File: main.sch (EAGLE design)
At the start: 4 parts, among them X1 1751248, X2 1751251

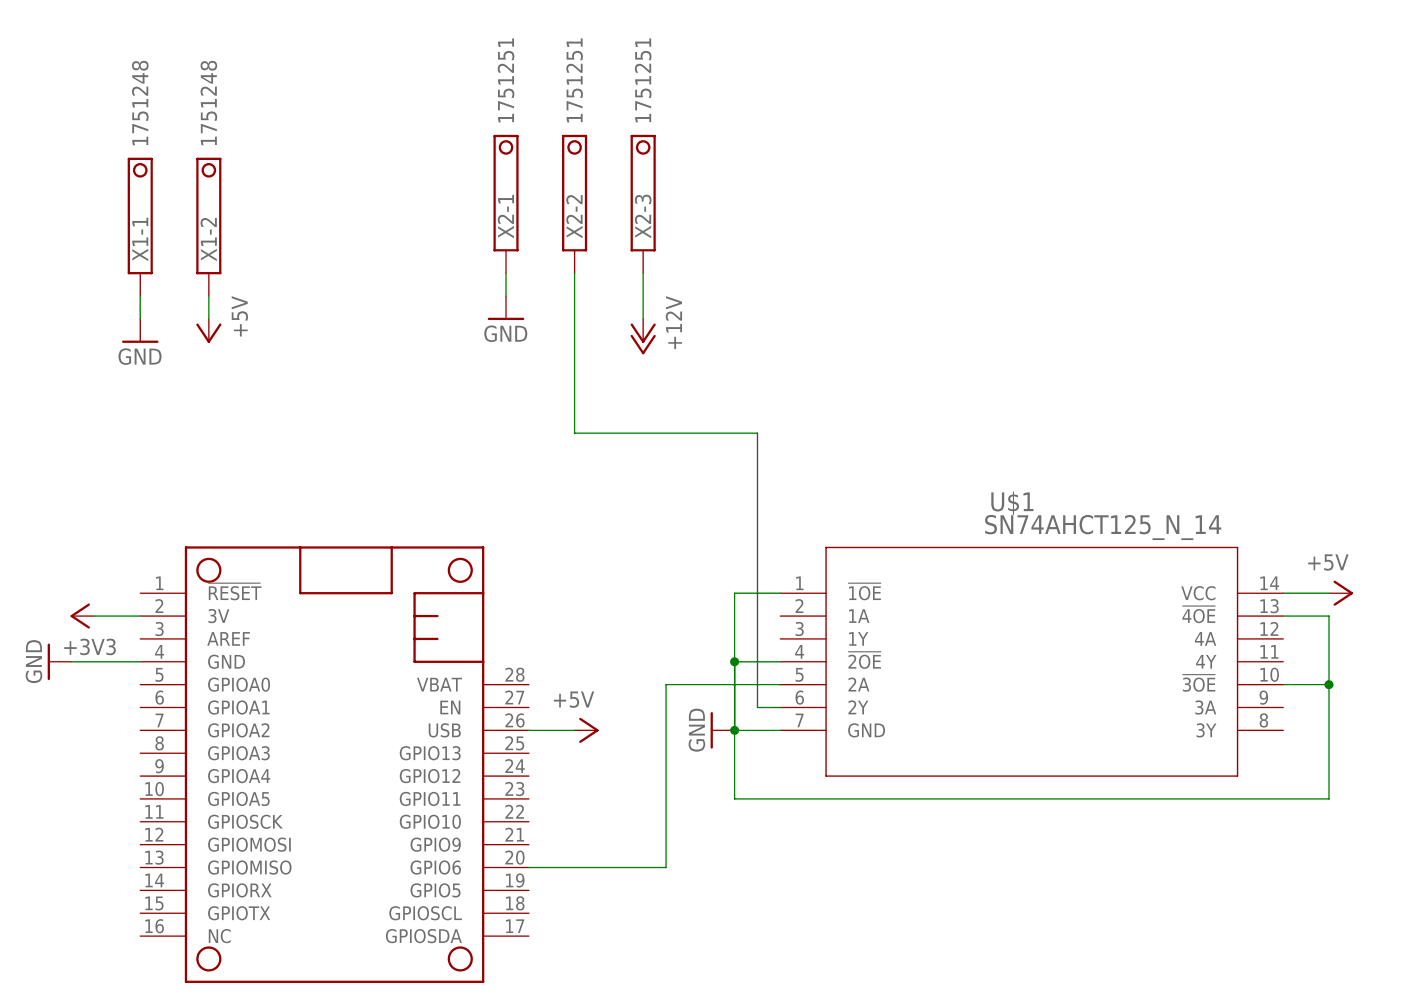
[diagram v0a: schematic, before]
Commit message: v2
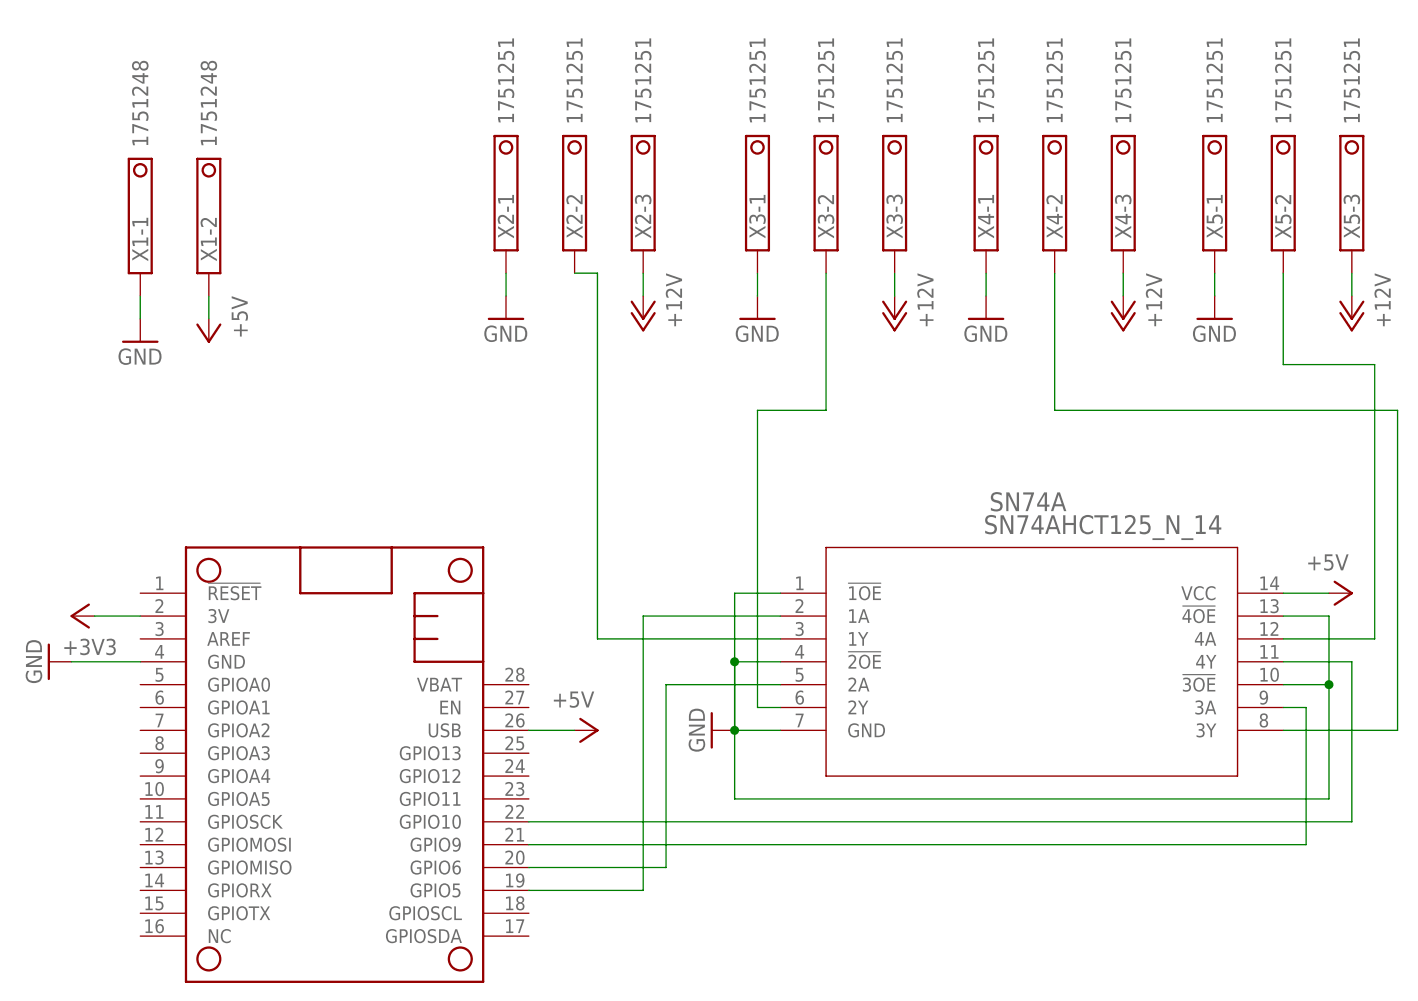
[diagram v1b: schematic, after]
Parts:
- added X3, X4, X5: 1751251, con-phoenix-350:1751251
- renumbered U$1 to SN74A
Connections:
- net LDATA renamed LDATA2
- removed net HDATA: SN74A.2Y, X2-2.K
- new net HDATA1: SN74A.1Y, X2-2.K
- new net HDATA2: SN74A.2Y, X3-2.K
- new net HDATA3: SN74A.3Y, X4-2.K
- new net HDATA4: SN74A.4A, X5-2.K
- new net LDATA1: MS1.GPIO5, SN74A.1A
- new net LDATA3: MS1.GPIO9, SN74A.3A
- new net LDATA4: MS1.GPIO10, SN74A.4Y
- net +12V: now also X3-3.K, X4-3.K, X5-3.K
- net GND: now also X3-1.K, X4-1.K, X5-1.K
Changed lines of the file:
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@@
 </variantdefs>
 <classes>
-<class number="0" name="default" width="0.381" drill="0">
+<class number="0" name="default" width="0.762" drill="0">
 <clearance class="0" value="0.3048"/>
 </class>
@@
 <parts>
 <part name="MS1" library="adafruit" deviceset="FEATHERWING" device="_NODIM"/>
-<part name="U$1" library="SN74AHCT125N" deviceset="SN74AHCT125_N_14" device=""/>
+<part name="SN74A" library="SN74AHCT125N" deviceset="SN74AHCT125_N_14" device=""/>
 <part name="GND2" library="supply1" deviceset="GND" device=""/>
 <part name="GND3" library="supply1" deviceset="GND" device=""/>
@@
 <part name="P+3" library="supply1" deviceset="+5V" device=""/>
 <part name="P+4" library="supply1" deviceset="+12V" device=""/>
+<part name="X3" library="con-phoenix-350" deviceset="1751251" device=""/>
+<part name="X4" library="con-phoenix-350" deviceset="1751251" device=""/>
+<part name="X5" library="con-phoenix-350" deviceset="1751251" device=""/>
+<part name="GND5" library="supply1" deviceset="GND" device=""/>
+<part name="GND6" library="supply1" deviceset="GND" device=""/>
+<part name="GND7" library="supply1" deviceset="GND" device=""/>
+<part name="P+5" library="supply1" deviceset="+12V" device=""/>
+<part name="P+6" library="supply1" deviceset="+12V" device=""/>
+<part name="P+7" library="supply1" deviceset="+12V" device=""/>
 </parts>
 <sheets>
@@
 <instances>
 <instance part="MS1" gate="G$1" x="-27.94" y="81.28" rot="R270"/>
-<instance part="U$1" gate="A" x="35.56" y="76.2"/>
+<instance part="SN74A" gate="A" x="35.56" y="76.2"/>
 <instance part="GND2" gate="1" x="-43.18" y="68.58" rot="R270"/>
 <instance part="GND3" gate="1" x="30.48" y="60.96" rot="R270"/>
@@
 <instance part="GND4" gate="1" x="7.62" y="106.68"/>
 <instance part="P+3" gate="1" x="101.6" y="76.2" rot="R270"/>
-<instance part="P+4" gate="1" x="22.86" y="104.14" rot="R180"/>
+<instance part="P+4" gate="1" x="22.86" y="106.68" rot="R180"/>
+<instance part="X3" gate="-1" x="35.56" y="114.3" rot="R90"/>
+<instance part="X3" gate="-2" x="43.18" y="114.3" rot="R90"/>
+<instance part="X3" gate="-3" x="50.8" y="114.3" rot="R90"/>
+<instance part="X4" gate="-1" x="60.96" y="114.3" rot="R90"/>
+<instance part="X4" gate="-2" x="68.58" y="114.3" rot="R90"/>
+<instance part="X4" gate="-3" x="76.2" y="114.3" rot="R90"/>
+<instance part="X5" gate="-1" x="86.36" y="114.3" rot="R90"/>
+<instance part="X5" gate="-2" x="93.98" y="114.3" rot="R90"/>
+<instance part="X5" gate="-3" x="101.6" y="114.3" rot="R90"/>
+<instance part="GND5" gate="1" x="35.56" y="106.68"/>
+<instance part="GND6" gate="1" x="60.96" y="106.68"/>
+<instance part="GND7" gate="1" x="86.36" y="106.68"/>
+<instance part="P+5" gate="1" x="50.8" y="106.68" rot="R180"/>
+<instance part="P+6" gate="1" x="76.2" y="106.68" rot="R180"/>
+<instance part="P+7" gate="1" x="101.6" y="106.68" rot="R180"/>
 </instances>
 <busses>
@@
 <segment>
 <pinref part="GND3" gate="1" pin="GND"/>
-<pinref part="U$1" gate="A" pin="GND"/>
+<pinref part="SN74A" gate="A" pin="GND"/>
 <wire x1="33.02" y1="60.96" x2="38.1" y2="60.96" width="0.1524" layer="91"/>
-<pinref part="U$1" gate="A" pin="!2OE"/>
+<pinref part="SN74A" gate="A" pin="!2OE"/>
 <wire x1="38.1" y1="68.58" x2="33.02" y2="68.58" width="0.1524" layer="91"/>
 <wire x1="33.02" y1="68.58" x2="33.02" y2="60.96" width="0.1524" layer="91"/>
-<pinref part="U$1" gate="A" pin="!1OE"/>
+<pinref part="SN74A" gate="A" pin="!1OE"/>
 <wire x1="38.1" y1="76.2" x2="33.02" y2="76.2" width="0.1524" layer="91"/>
 <wire x1="33.02" y1="76.2" x2="33.02" y2="68.58" width="0.1524" layer="91"/>
@@
 <wire x1="33.02" y1="53.34" x2="99.06" y2="53.34" width="0.1524" layer="91"/>
 <wire x1="99.06" y1="53.34" x2="99.06" y2="66.04" width="0.1524" layer="91"/>
-<pinref part="U$1" gate="A" pin="!3OE"/>
+<pinref part="SN74A" gate="A" pin="!3OE"/>
 <wire x1="93.98" y1="66.04" x2="99.06" y2="66.04" width="0.1524" layer="91"/>
 <wire x1="99.06" y1="66.04" x2="99.06" y2="73.66" width="0.1524" layer="91"/>
-<pinref part="U$1" gate="A" pin="!4OE"/>
+<pinref part="SN74A" gate="A" pin="!4OE"/>
 <wire x1="99.06" y1="73.66" x2="93.98" y2="73.66" width="0.1524" layer="91"/>
 <junction x="33.02" y="68.58"/>
@@
 <wire x1="7.62" y1="109.22" x2="7.62" y2="111.76" width="0.1524" layer="91"/>
 </segment>
+<segment>
+<pinref part="X3" gate="-1" pin="K"/>
+<pinref part="GND5" gate="1" pin="GND"/>
+<wire x1="35.56" y1="111.76" x2="35.56" y2="109.22" width="0.1524" layer="91"/>
+</segment>
+<segment>
+<pinref part="X4" gate="-1" pin="K"/>
+<pinref part="GND6" gate="1" pin="GND"/>
+<wire x1="60.96" y1="111.76" x2="60.96" y2="109.22" width="0.1524" layer="91"/>
+</segment>
+<segment>
+<pinref part="X5" gate="-1" pin="K"/>
+<pinref part="GND7" gate="1" pin="GND"/>
+<wire x1="86.36" y1="111.76" x2="86.36" y2="109.22" width="0.1524" layer="91"/>
+</segment>
 </net>
 <net name="+3V3" class="0">
@@
 </segment>
 <segment>
-<pinref part="U$1" gate="A" pin="VCC"/>
+<pinref part="SN74A" gate="A" pin="VCC"/>
 <pinref part="P+3" gate="1" pin="+5V"/>
 <wire x1="93.98" y1="76.2" x2="99.06" y2="76.2" width="0.1524" layer="91"/>
@@
 </segment>
 </net>
-<net name="LDATA" class="0">
+<net name="LDATA2" class="0">
 <segment>
 <pinref part="MS1" gate="G$1" pin="GPIO6"/>
 <wire x1="10.16" y1="45.72" x2="25.4" y2="45.72" width="0.1524" layer="91"/>
 <wire x1="25.4" y1="45.72" x2="25.4" y2="66.04" width="0.1524" layer="91"/>
-<pinref part="U$1" gate="A" pin="2A"/>
+<pinref part="SN74A" gate="A" pin="2A"/>
 <wire x1="25.4" y1="66.04" x2="38.1" y2="66.04" width="0.1524" layer="91"/>
 </segment>
@@
 <pinref part="P+4" gate="1" pin="+12V"/>
 <pinref part="X2" gate="-3" pin="K"/>
-<wire x1="22.86" y1="106.68" x2="22.86" y2="111.76" width="0.1524" layer="91"/>
-</segment>
-</net>
-<net name="HDATA" class="0">
-<segment>
-<pinref part="U$1" gate="A" pin="2Y"/>
+<wire x1="22.86" y1="109.22" x2="22.86" y2="111.76" width="0.1524" layer="91"/>
+</segment>
+<segment>
+<pinref part="X3" gate="-3" pin="K"/>
+<pinref part="P+5" gate="1" pin="+12V"/>
+<wire x1="50.8" y1="111.76" x2="50.8" y2="109.22" width="0.1524" layer="91"/>
+</segment>
+<segment>
+<pinref part="X4" gate="-3" pin="K"/>
+<pinref part="P+6" gate="1" pin="+12V"/>
+<wire x1="76.2" y1="111.76" x2="76.2" y2="109.22" width="0.1524" layer="91"/>
+</segment>
+<segment>
+<pinref part="X5" gate="-3" pin="K"/>
+<pinref part="P+7" gate="1" pin="+12V"/>
+<wire x1="101.6" y1="111.76" x2="101.6" y2="109.22" width="0.1524" layer="91"/>
+</segment>
+</net>
+<net name="LDATA1" class="0">
+<segment>
+<pinref part="MS1" gate="G$1" pin="GPIO5"/>
+<wire x1="10.16" y1="43.18" x2="22.86" y2="43.18" width="0.1524" layer="91"/>
+<wire x1="22.86" y1="43.18" x2="22.86" y2="73.66" width="0.1524" layer="91"/>
+<pinref part="SN74A" gate="A" pin="1A"/>
+<wire x1="22.86" y1="73.66" x2="38.1" y2="73.66" width="0.1524" layer="91"/>
+</segment>
+</net>
+<net name="LDATA3" class="0">
+<segment>
+<pinref part="MS1" gate="G$1" pin="GPIO9"/>
+<wire x1="10.16" y1="48.26" x2="96.52" y2="48.26" width="0.1524" layer="91"/>
+<wire x1="96.52" y1="48.26" x2="96.52" y2="63.5" width="0.1524" layer="91"/>
+<pinref part="SN74A" gate="A" pin="3A"/>
+<wire x1="96.52" y1="63.5" x2="93.98" y2="63.5" width="0.1524" layer="91"/>
+</segment>
+</net>
+<net name="HDATA3" class="0">
+<segment>
+<pinref part="SN74A" gate="A" pin="3Y"/>
+<wire x1="93.98" y1="60.96" x2="106.68" y2="60.96" width="0.1524" layer="91"/>
+<wire x1="106.68" y1="60.96" x2="106.68" y2="96.52" width="0.1524" layer="91"/>
+<wire x1="106.68" y1="96.52" x2="68.58" y2="96.52" width="0.1524" layer="91"/>
+<pinref part="X4" gate="-2" pin="K"/>
+<wire x1="68.58" y1="96.52" x2="68.58" y2="111.76" width="0.1524" layer="91"/>
+</segment>
+</net>
+<net name="LDATA4" class="0">
+<segment>
+<pinref part="MS1" gate="G$1" pin="GPIO10"/>
+<wire x1="10.16" y1="50.8" x2="101.6" y2="50.8" width="0.1524" layer="91"/>
+<wire x1="101.6" y1="50.8" x2="101.6" y2="68.58" width="0.1524" layer="91"/>
+<pinref part="SN74A" gate="A" pin="4Y"/>
+<wire x1="101.6" y1="68.58" x2="93.98" y2="68.58" width="0.1524" layer="91"/>
+</segment>
+</net>
+<net name="HDATA4" class="0">
+<segment>
+<pinref part="SN74A" gate="A" pin="4A"/>
+<wire x1="93.98" y1="71.12" x2="104.14" y2="71.12" width="0.1524" layer="91"/>
+<wire x1="104.14" y1="71.12" x2="104.14" y2="101.6" width="0.1524" layer="91"/>
+<wire x1="104.14" y1="101.6" x2="93.98" y2="101.6" width="0.1524" layer="91"/>
+<pinref part="X5" gate="-2" pin="K"/>
+<wire x1="93.98" y1="101.6" x2="93.98" y2="111.76" width="0.1524" layer="91"/>
+</segment>
+</net>
+<net name="HDATA1" class="0">
+<segment>
+<pinref part="X2" gate="-2" pin="K"/>
+<wire x1="15.24" y1="111.76" x2="17.78" y2="111.76" width="0.1524" layer="91"/>
+<wire x1="17.78" y1="111.76" x2="17.78" y2="71.12" width="0.1524" layer="91"/>
+<pinref part="SN74A" gate="A" pin="1Y"/>
+<wire x1="17.78" y1="71.12" x2="38.1" y2="71.12" width="0.1524" layer="91"/>
+</segment>
+</net>
+<net name="HDATA2" class="0">
+<segment>
+<pinref part="SN74A" gate="A" pin="2Y"/>
 <wire x1="38.1" y1="63.5" x2="35.56" y2="63.5" width="0.1524" layer="91"/>
-<wire x1="35.56" y1="63.5" x2="35.56" y2="93.98" width="0.1524" layer="91"/>
-<wire x1="35.56" y1="93.98" x2="15.24" y2="93.98" width="0.1524" layer="91"/>
-<pinref part="X2" gate="-2" pin="K"/>
-<wire x1="15.24" y1="93.98" x2="15.24" y2="111.76" width="0.1524" layer="91"/>
-</segment>
-</net>
+<wire x1="35.56" y1="63.5" x2="35.56" y2="96.52" width="0.1524" layer="91"/>
+<pinref part="X3" gate="-2" pin="K"/>
+<wire x1="35.56" y1="96.52" x2="43.18" y2="96.52" width="0.1524" layer="91"/>
+<wire x1="43.18" y1="96.52" x2="43.18" y2="111.76" width="0.1524" layer="91"/>
+</segment>
+</net>
